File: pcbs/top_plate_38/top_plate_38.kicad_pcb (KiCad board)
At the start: 2 copper layers, 115.6 x 95.3 mm, 6 parts

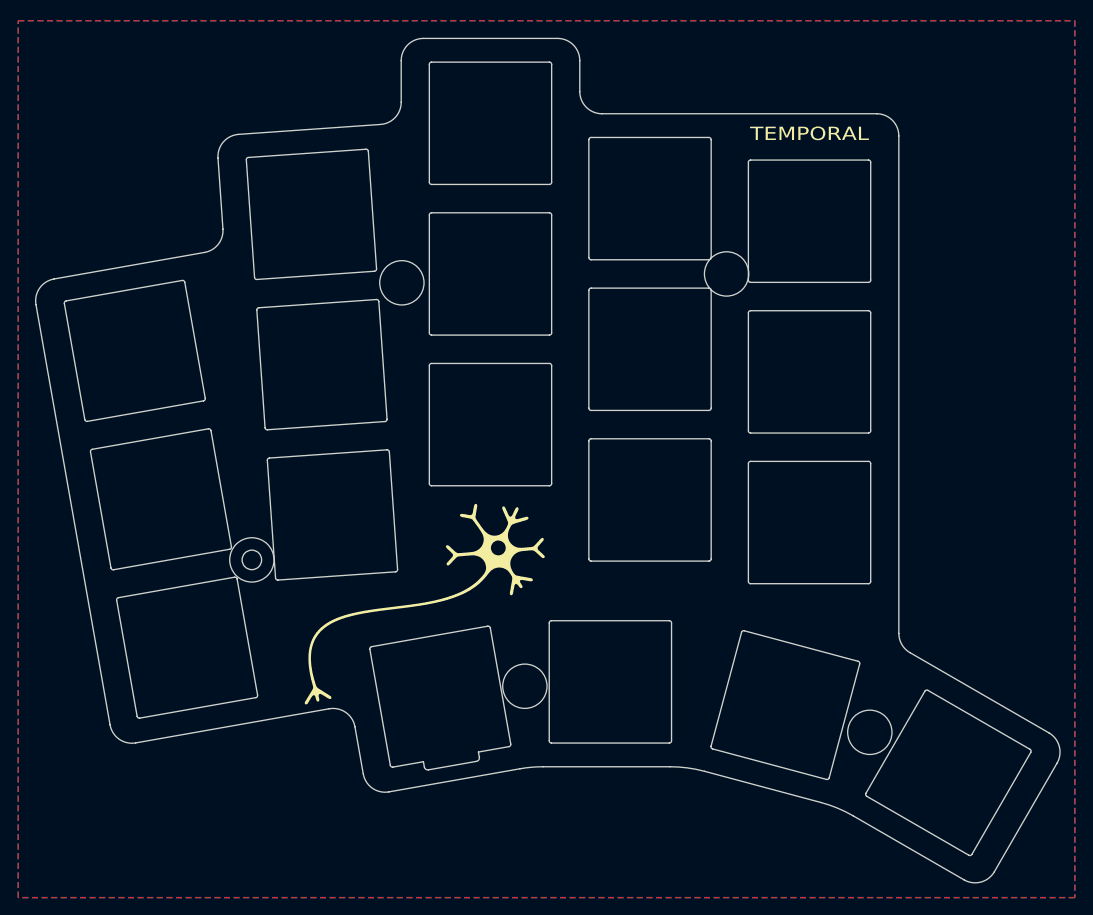
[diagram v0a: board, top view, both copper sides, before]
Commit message: update generated files
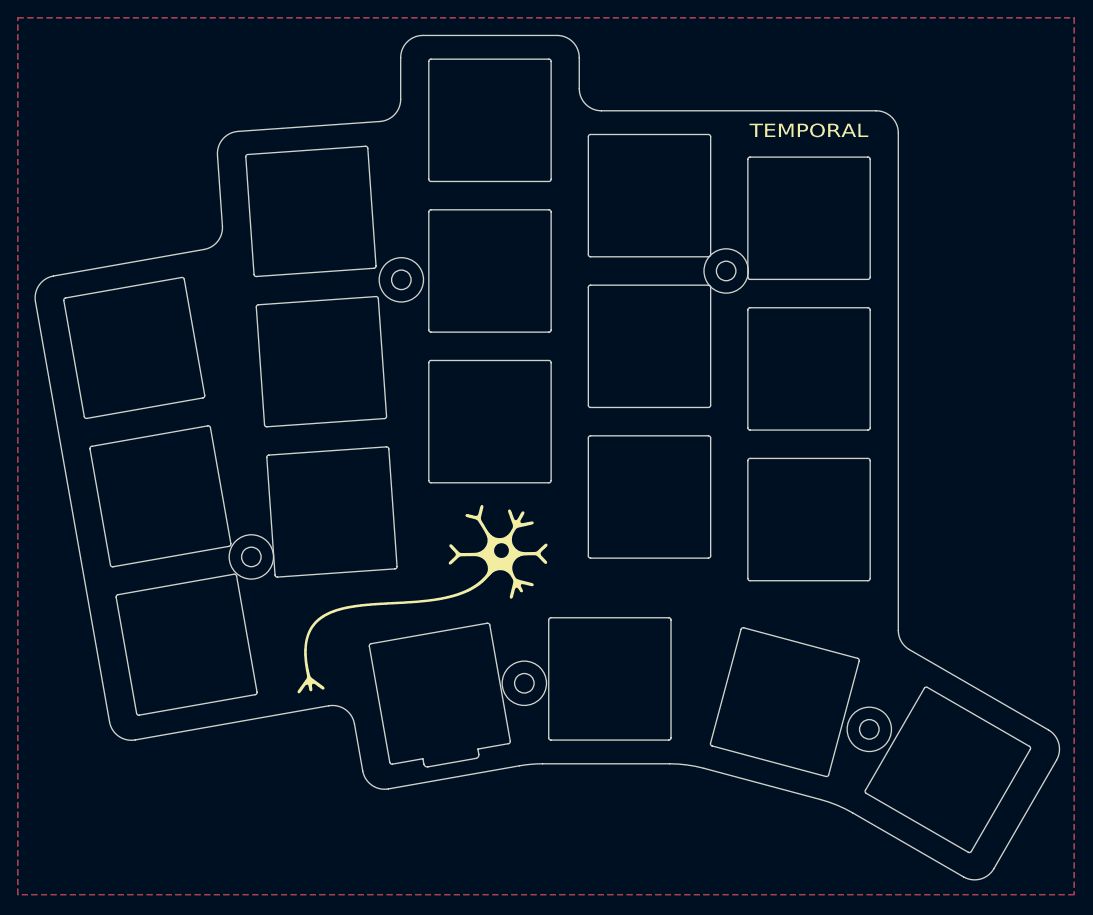
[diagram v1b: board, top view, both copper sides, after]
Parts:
- moved G1 0.34 mm to (92.8, 83.0), turned to 0 degrees
- moved MH3 0.34 mm to (143.2, 97.7)
- moved MH4 0.34 mm to (104.3, 92.5)
- moved MH5 0.34 mm to (73.5, 78.3)
- moved MH1 0.34 mm to (90.4, 47.0)
- moved MH2 0.34 mm to (127.1, 46.0)
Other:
- outline, holes or cut-outs redrawn

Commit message: update generated files
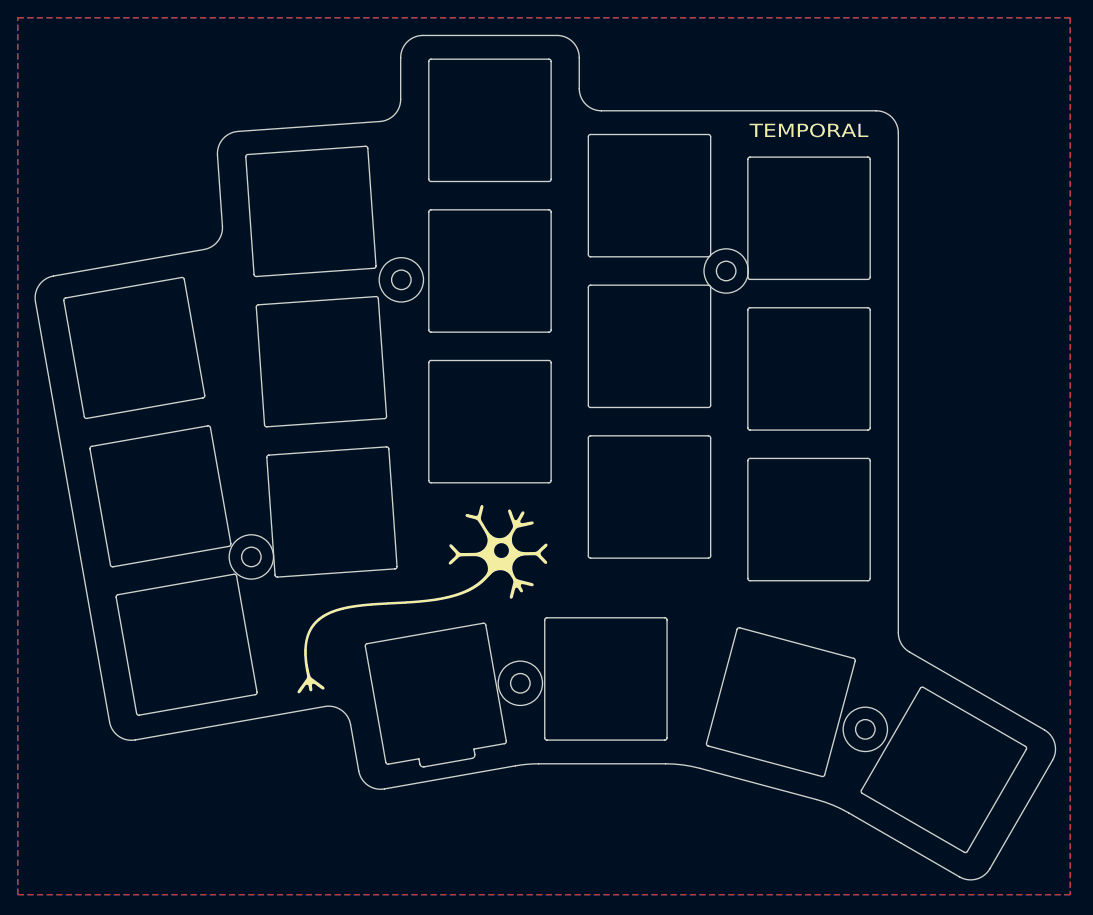
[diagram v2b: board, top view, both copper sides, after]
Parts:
- moved MH3 0.45 mm to (142.8, 97.7)
- moved MH4 0.45 mm to (103.9, 92.5)
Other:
- board size 115.6 x 95.3 mm -> 115.1 x 95.3 mm
